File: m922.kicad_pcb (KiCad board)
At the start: 2 copper layers, 54.6 x 40 mm, 12 parts, among them J1 Conn_01x02, J2 Conn_01x02, J3 Conn_01x02, J4 Conn_01x02, J5 Conn_01x02, J6 Conn_01x02

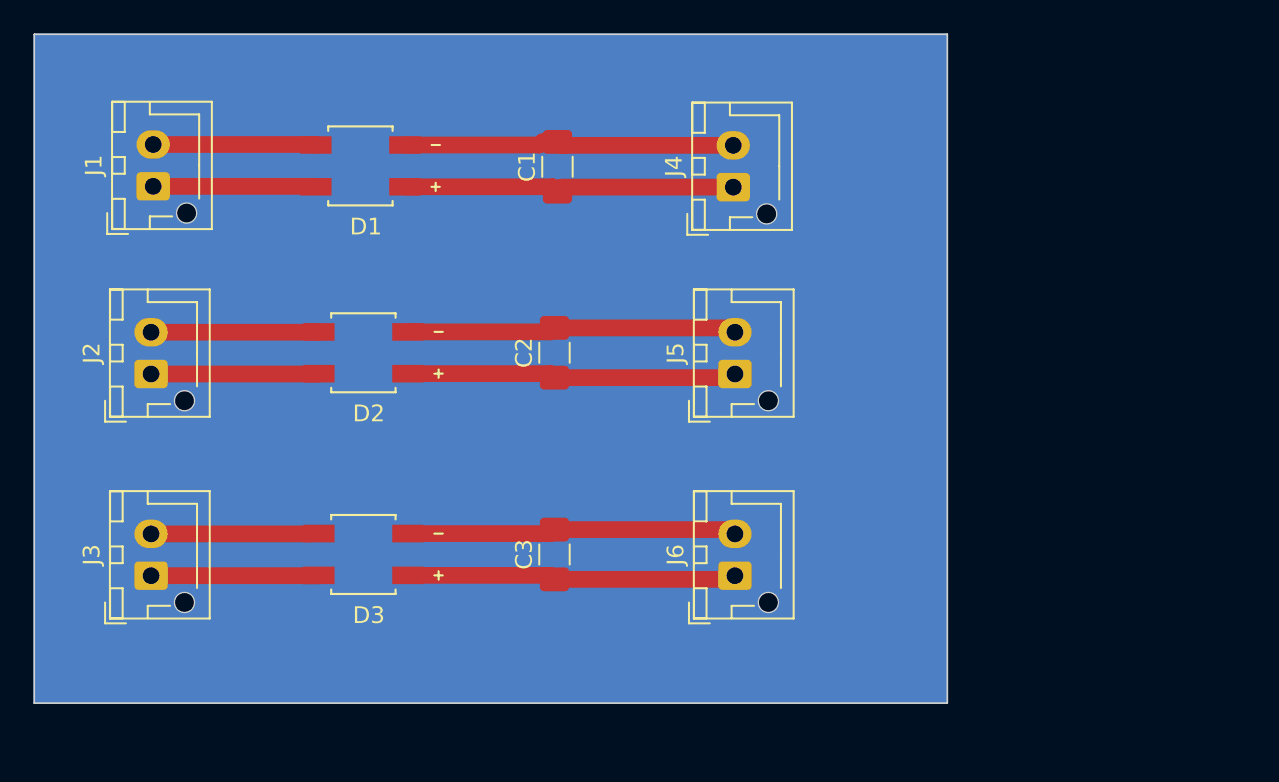
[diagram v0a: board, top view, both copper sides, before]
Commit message: 試作第一案
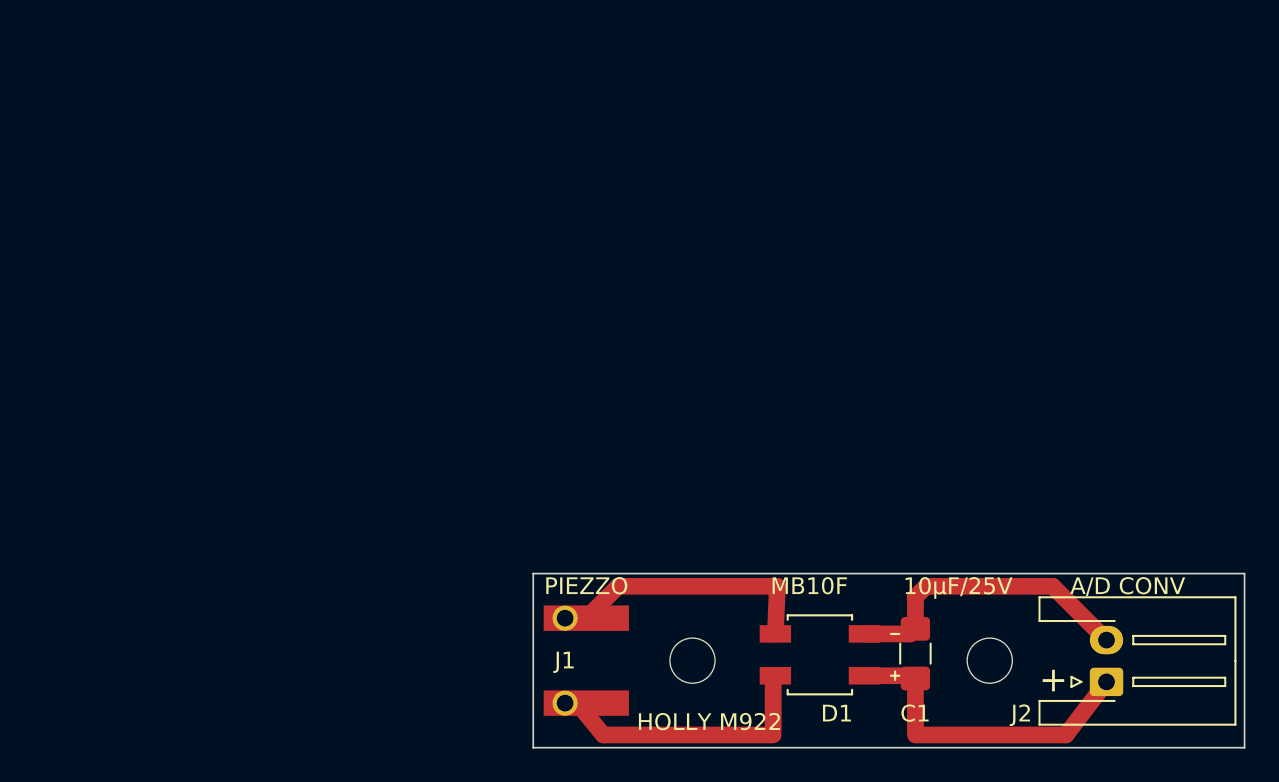
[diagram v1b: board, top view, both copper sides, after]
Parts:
- removed C2, C3: 10μF/25V, Capacitor_SMD:C_1206_3216Metric_Pad1.42x1.75mm_HandSolder
- removed D2, D3: MB10F-13, DIOB_MB10F-13
- removed J3, J4, J5, J6: Conn_01x02, Connector_JST:JST_XH_B2B-XH-AM_1x02_P2.50mm_Vertical
- added ?: , , F.Cu at (122.7, 88.6)
- added ?: , , F.Cu at (130.0, 89.2)
- added ?: , , F.Cu at (120.7, 96.5)
- added REF**: MountingHole_2.7mm, MountingHole:MountingHole_2.7mm, F.Cu at (121.9, 85.7)
- added REF**: MountingHole_2.7mm, MountingHole:MountingHole_2.7mm, F.Cu at (139.7, 85.7)
- C1: value 10μF/25V (P-14741) -> 10μF/25V
- D1: value MB10F-13 -> MB10F
- J1: value Conn_01x02 -> PIEZZO; footprint Connector_JST:JST_XH_B2B-XH-AM_1x02_P2.50mm_Vertical -> HOLLY:LDT0-028K_MID
- J2: value Conn_01x02 -> A/D CONV; footprint Connector_JST:JST_XH_B2B-XH-AM_1x02_P2.50mm_Vertical -> Connector_JST:JST_XH_S2B-XH-A-1_1x02_P2.50mm_Horizontal
- moved J2 60.0 mm to (146.7, 87.0)
- moved D1 40.1 mm to (129.5, 85.4)
- moved C1 36.1 mm to (135.3, 85.3)
- moved J1 34.8 mm to (113.0, 83.2), turned to 0 degrees
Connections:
- C1 pad 2: GND -> Net-(C1-Pad2)
- D1 pad 3: GND -> Net-(C1-Pad2)
- J1 pad 2: Net-(D1-Pad4) -> Net-(D1-Pad2)
- J2 pad 1: Net-(D2-Pad2) -> Net-(C1-Pad1)
- J2 pad 2: Net-(D2-Pad4) -> Net-(C1-Pad2)
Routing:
- net GND: track 59.3 -> 0.00 mm
- net Net-(C3-Pad1): track 19.8 -> 0.00 mm
- net Net-(C2-Pad1): track 19.8 -> 0.00 mm
- net Net-(C1-Pad2): track 0.00 -> 18.1 mm
- net Net-(D3-Pad2): track 10.0 -> 0.00 mm
- net Net-(D2-Pad4): track 10.0 -> 0.00 mm
- net Net-(D2-Pad2): track 10.0 -> 0.00 mm
- net Net-(D3-Pad4): track 9.48 -> 0.00 mm
- net Net-(D1-Pad2): track 9.75 -> 15.3 mm
- net Net-(D1-Pad4): track 9.75 -> 15.1 mm
- net Net-(C1-Pad1): track 19.9 -> 19.2 mm
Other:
- board size 54.6 x 40 mm -> 42.5 x 10.4 mm
- board text added: "+"
- board text added: "HOLLY M922 2109A"
